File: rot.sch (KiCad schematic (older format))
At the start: 34 parts, among them J3 543630489, J4 M20-7830642, U2 W25Q32JVSSIQ_TR, U3 W25Q32JVSSIQ_TR, U4 W25Q32JVSSIQ_TR, U5 W25Q32JVSSIQ_TR

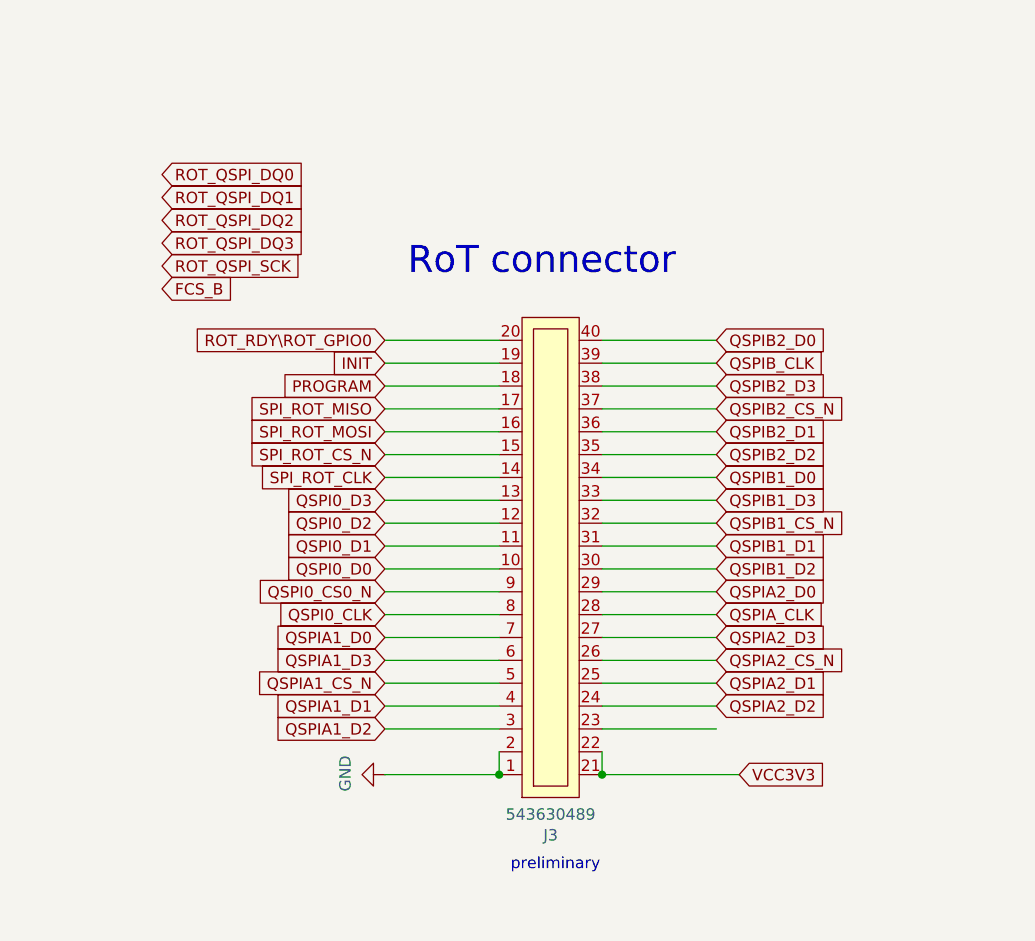
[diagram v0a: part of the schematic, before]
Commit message: Reconnected interfaces
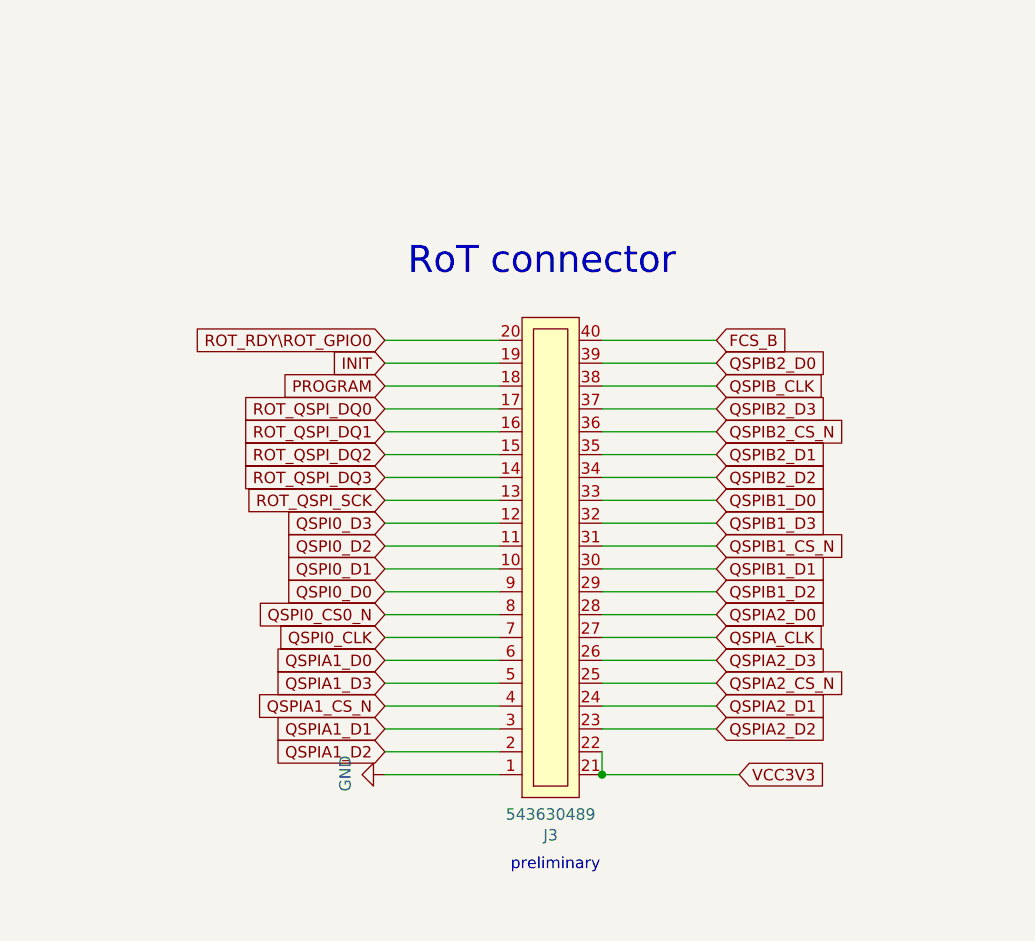
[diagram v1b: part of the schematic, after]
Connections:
- net SPI_ROT_CLK is gone; now on net ROT_QSPI_DQ3: J3.14
- net SPI_ROT_CS_N is gone; now on net ROT_QSPI_DQ2: J3.15
- net SPI_ROT_MISO is gone; now on net ROT_QSPI_DQ0: J3.17
- net SPI_ROT_MOSI is gone; now on net ROT_QSPI_DQ1: J3.16
- net FCS_B: now also J3.40
- net GND: no longer J3.2
- net QSPI0_CLK: now also J3.7; no longer J3.8
- net QSPI0_CS0_N: now also J3.8; no longer J3.9
- net QSPI0_D0: now also J3.9; no longer J3.10
- net QSPI0_D1: now also J3.10; no longer J3.11
- net QSPI0_D2: now also J3.11; no longer J3.12
- net QSPI0_D3: now also J3.12; no longer J3.13
- net QSPIA1_CS_N: now also J3.4; no longer J3.5
- net QSPIA1_D0: now also J3.6; no longer J3.7
- net QSPIA1_D1: now also J3.3; no longer J3.4
- net QSPIA1_D2: now also J3.2; no longer J3.3
- net QSPIA1_D3: now also J3.5; no longer J3.6
- net QSPIA2_CS_N: now also J3.25; no longer J3.26
- net QSPIA2_D0: now also J3.28; no longer J3.29
- net QSPIA2_D1: now also J3.24; no longer J3.25
- net QSPIA2_D2: now also J3.23; no longer J3.24
- net QSPIA2_D3: now also J3.26; no longer J3.27
- net QSPIA_CLK: now also J3.27; no longer J3.28
- net QSPIB1_CS_N: now also J3.31; no longer J3.32
- net QSPIB1_D0: now also J3.33; no longer J3.34
- net QSPIB1_D1: now also J3.30; no longer J3.31
- net QSPIB1_D2: now also J3.29; no longer J3.30
- net QSPIB1_D3: now also J3.32; no longer J3.33
- net QSPIB2_CS_N: now also J3.36; no longer J3.37
- net QSPIB2_D0: now also J3.39; no longer J3.40
- net QSPIB2_D1: now also J3.35; no longer J3.36
- net QSPIB2_D2: now also J3.34; no longer J3.35
- net QSPIB2_D3: now also J3.37; no longer J3.38
- net QSPIB_CLK: now also J3.38; no longer J3.39
- net ROT_QSPI_SCK: now also J3.13
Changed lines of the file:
@@
 Comment4 ""
 $EndDescr
-$Comp
-L artix-dc-scm:543630489 J3
-U 1 1 6268C044
-P 8925 6775
-F 0 "J3" H 8950 6790 50  0000 C CNN
-F 1 "543630489" H 8950 6699 50  0000 C CNN
-F 2 "artix-dc-scm-footprints:543630489" H 8675 4425 50  0001 C CNN
-F 3 "https://www.molex.com/pdm_docs/sd/543630489_sd.pdf" H 9175 4475 50  0001 C CNN
-	1    8925 6775
-	1    0    0    1
-$EndComp
+Wire Wire Line
+	8725 6425 8225 6425
 Wire Wire Line
 	8725 6325 8225 6325
-Wire Wire Line
-	8725 6225 8225 6225
 Text GLabel 1950 2550 0    50   Input ~ 0
 QSPIA1_CS_N
@@
 Text Notes 1475 1475 0    50   ~ 0
 One or typically two flash devices used to contain the BIOS firmware image
-Text GLabel 8225 5225 0    50   Input ~ 0
-SPI_ROT_CLK
-Text GLabel 8225 5125 0    50   Input ~ 0
-SPI_ROT_CS_N
-Text GLabel 8225 5025 0    50   Input ~ 0
-SPI_ROT_MOSI
-Text GLabel 8225 4925 0    50   Input ~ 0
-SPI_ROT_MISO
+Wire Wire Line
+	8725 6225 8225 6225
 Wire Wire Line
 	8725 6125 8225 6125
-Wire Wire Line
-	8725 6025 8225 6025
+Text GLabel 8225 6225 0    50   Input ~ 0
+QSPIA1_CS_N
+Text GLabel 9675 5925 2    50   Input ~ 0
+QSPIA_CLK
+Text GLabel 8225 6025 0    50   Input ~ 0
+QSPIA1_D0
+Text GLabel 8225 6425 0    50   Input ~ 0
+QSPIA1_D2
 Text GLabel 8225 6125 0    50   Input ~ 0
-QSPIA1_CS_N
+QSPIA1_D3
+Text GLabel 9675 6125 2    50   Input ~ 0
+QSPIA2_CS_N
 Text GLabel 9675 5825 2    50   Input ~ 0
-QSPIA_CLK
+QSPIA2_D0
+Text GLabel 9675 6325 2    50   Input ~ 0
+QSPIA2_D2
+Text GLabel 9675 6025 2    50   Input ~ 0
+QSPIA2_D3
+Text GLabel 9675 5525 2    50   Input ~ 0
+QSPIB1_CS_N
+Text GLabel 9675 4825 2    50   Input ~ 0
+QSPIB_CLK
+Text GLabel 9675 5325 2    50   Input ~ 0
+QSPIB1_D0
+Text GLabel 9675 5725 2    50   Input ~ 0
+QSPIB1_D2
+Text GLabel 9675 5425 2    50   Input ~ 0
+QSPIB1_D3
+Text GLabel 9675 5025 2    50   Input ~ 0
+QSPIB2_CS_N
+Text GLabel 9675 4725 2    50   Input ~ 0
+QSPIB2_D0
+Text GLabel 9675 5225 2    50   Input ~ 0
+QSPIB2_D2
+Text GLabel 9675 4925 2    50   Input ~ 0
+QSPIB2_D3
+Text GLabel 8225 6325 0    50   Input ~ 0
+QSPIA1_D1
+Text GLabel 9675 6225 2    50   Input ~ 0
+QSPIA2_D1
+Text GLabel 9675 5625 2    50   Input ~ 0
+QSPIB1_D1
+Text GLabel 9675 5125 2    50   Input ~ 0
+QSPIB2_D1
 Text GLabel 8225 5925 0    50   Input ~ 0
-QSPIA1_D0
-Text GLabel 8225 6325 0    50   Input ~ 0
-QSPIA1_D2
-Text GLabel 8225 6025 0    50   Input ~ 0
-QSPIA1_D3
-Text GLabel 9675 6025 2    50   Input ~ 0
-QSPIA2_CS_N
-Text GLabel 9675 5725 2    50   Input ~ 0
-QSPIA2_D0
-Text GLabel 9675 6225 2    50   Input ~ 0
-QSPIA2_D2
-Text GLabel 9675 5925 2    50   Input ~ 0
-QSPIA2_D3
-Text GLabel 9675 5425 2    50   Input ~ 0
-QSPIB1_CS_N
-Text GLabel 9675 4725 2    50   Input ~ 0
-QSPIB_CLK
-Text GLabel 9675 5225 2    50   Input ~ 0
-QSPIB1_D0
-Text GLabel 9675 5625 2    50   Input ~ 0
-QSPIB1_D2
-Text GLabel 9675 5325 2    50   Input ~ 0
-QSPIB1_D3
-Text GLabel 9675 4925 2    50   Input ~ 0
-QSPIB2_CS_N
-Text GLabel 9675 4625 2    50   Input ~ 0
-QSPIB2_D0
-Text GLabel 9675 5125 2    50   Input ~ 0
-QSPIB2_D2
-Text GLabel 9675 4825 2    50   Input ~ 0
-QSPIB2_D3
-Text GLabel 8225 6225 0    50   Input ~ 0
-QSPIA1_D1
-Text GLabel 9675 6125 2    50   Input ~ 0
-QSPIA2_D1
-Text GLabel 9675 5525 2    50   Input ~ 0
-QSPIB1_D1
-Text GLabel 9675 5025 2    50   Input ~ 0
-QSPIB2_D1
+QSPI0_CLK
 Text GLabel 8225 5825 0    50   Input ~ 0
-QSPI0_CLK
+QSPI0_CS0_N
 Text GLabel 8225 5725 0    50   Input ~ 0
-QSPI0_CS0_N
+QSPI0_D0
 Text GLabel 8225 5625 0    50   Input ~ 0
-QSPI0_D0
+QSPI0_D1
 Text GLabel 8225 5525 0    50   Input ~ 0
-QSPI0_D1
+QSPI0_D2
 Text GLabel 8225 5425 0    50   Input ~ 0
-QSPI0_D2
-Text GLabel 8225 5325 0    50   Input ~ 0
 QSPI0_D3
 Wire Wire Line
-	8225 5925 8725 5925
+	8225 6025 8725 6025
+Wire Wire Line
+	8725 5925 8225 5925
 Wire Wire Line
 	8725 5825 8225 5825
@@
 	8725 5625 8225 5625
 Wire Wire Line
+	8725 5425 8225 5425
+Wire Wire Line
+	8725 5225 8225 5225
+Wire Wire Line
+	8725 5125 8225 5125
+Wire Wire Line
+	8725 5025 8225 5025
+Wire Wire Line
+	9175 5825 9675 5825
+Wire Wire Line
+	9175 5725 9675 5725
+Wire Wire Line
+	9175 5625 9675 5625
+Wire Wire Line
+	9175 5525 9675 5525
+Wire Wire Line
+	9175 5325 9675 5325
+Wire Wire Line
+	9175 5225 9675 5225
+Wire Wire Line
+	9175 5125 9675 5125
+Wire Wire Line
+	9175 5025 9675 5025
+Wire Wire Line
+	8725 4925 8225 4925
+Wire Wire Line
+	9175 5925 9675 5925
+Wire Wire Line
+	9175 5425 9675 5425
+Wire Wire Line
+	9175 4925 9675 4925
+Wire Wire Line
 	8725 5525 8225 5525
-Wire Wire Line
-	8725 5325 8225 5325
-Wire Wire Line
-	8725 5225 8225 5225
-Wire Wire Line
-	8725 5125 8225 5125
-Wire Wire Line
-	8725 5025 8225 5025
-Wire Wire Line
-	9175 5825 9675 5825
-Wire Wire Line
-	9175 5725 9675 5725
-Wire Wire Line
-	9175 5625 9675 5625
-Wire Wire Line
-	9175 5525 9675 5525
-Wire Wire Line
-	9175 5325 9675 5325
-Wire Wire Line
-	9175 5225 9675 5225
-Wire Wire Line
-	9175 5125 9675 5125
-Wire Wire Line
-	9175 5025 9675 5025
-Wire Wire Line
-	8725 4925 8225 4925
-Wire Wire Line
-	9175 5925 9675 5925
-Wire Wire Line
-	9175 5425 9675 5425
-Wire Wire Line
-	9175 4925 9675 4925
-Wire Wire Line
-	8725 5425 8225 5425
 Wire Wire Line
 	9675 6325 9175 6325
@@
 $EndComp
 Wire Wire Line
-	8725 6425 8725 6525
-Connection ~ 8725 6525
-Wire Wire Line
 	9175 6525 9775 6525
 Wire Wire Line
 	9175 6425 9175 6525
 Connection ~ 9175 6525
-Text GLabel 7250 3900 2    50   Input ~ 0
+$Comp
+L artix-dc-scm:543630489 J3
+U 1 1 6268C044
+P 8925 6775
+F 0 "J3" H 8950 6790 50  0000 C CNN
+F 1 "543630489" H 8950 6699 50  0000 C CNN
+F 2 "artix-dc-scm-footprints:543630489" H 8675 4425 50  0001 C CNN
+F 3 "https://www.molex.com/pdm_docs/sd/543630489_sd.pdf" H 9175 4475 50  0001 C CNN
+	1    8925 6775
+	1    0    0    1
+$EndComp
+Text GLabel 9675 4625 2    50   Input ~ 0
+FCS_B
+Text GLabel 8225 5325 0    50   Input ~ 0
+ROT_QSPI_SCK
+Text GLabel 8225 5225 0    50   Input ~ 0
+ROT_QSPI_DQ3
+Text GLabel 8225 5125 0    50   Input ~ 0
+ROT_QSPI_DQ2
+Text GLabel 8225 5025 0    50   Input ~ 0
+ROT_QSPI_DQ1
+Text GLabel 8225 4925 0    50   Input ~ 0
 ROT_QSPI_DQ0
-Text GLabel 7250 4000 2    50   Input ~ 0
-ROT_QSPI_DQ1
-Text GLabel 7250 4100 2    50   Input ~ 0
-ROT_QSPI_DQ2
-Text GLabel 7250 4200 2    50   Input ~ 0
-ROT_QSPI_DQ3
-Text GLabel 7250 4300 2    50   Input ~ 0
-ROT_QSPI_SCK
-Text GLabel 7250 4400 2    50   Input ~ 0
-FCS_B
+Wire Wire Line
+	8725 5325 8225 5325
 $EndSCHEMATC
